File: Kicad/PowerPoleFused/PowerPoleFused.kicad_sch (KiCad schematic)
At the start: 6 parts, among them J1 Anderson powerpole, J2 Anderson powerpole, J3 Anderson powerpole, J4 Anderson powerpole, J5 Anderson powerpole, J6 Anderson powerpole

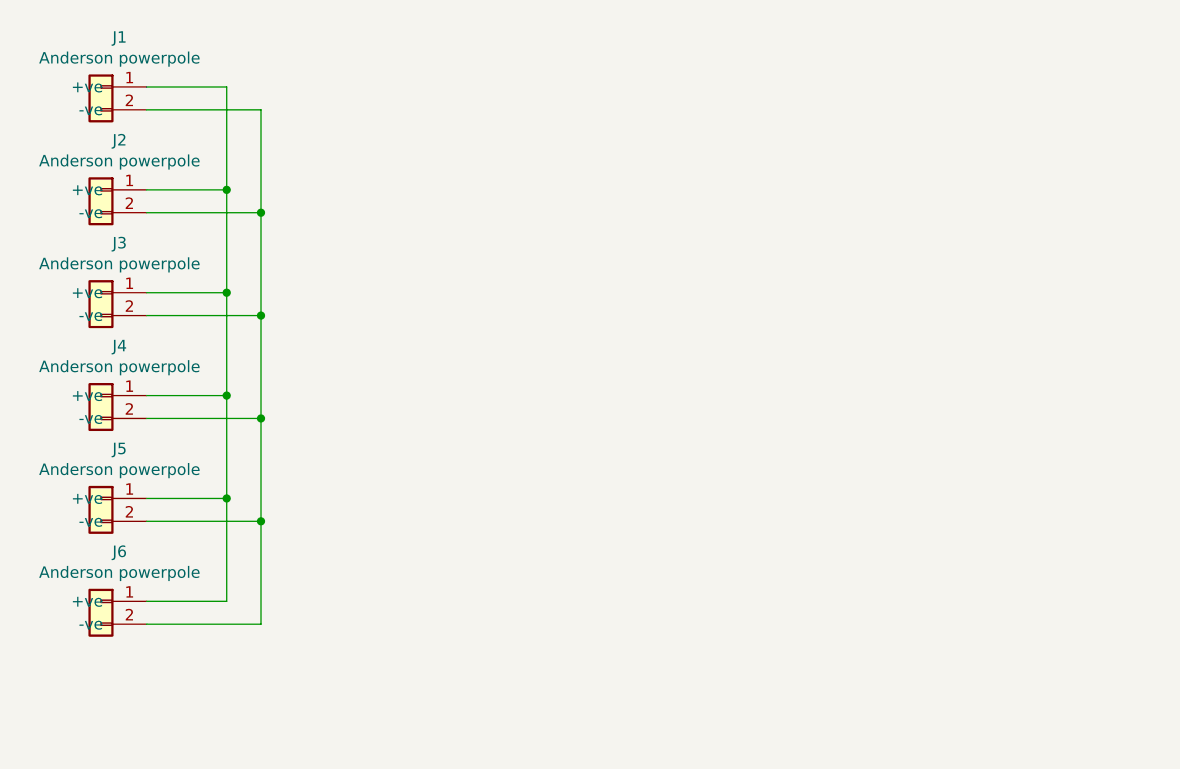
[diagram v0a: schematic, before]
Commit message: Laid out board 1st attempt
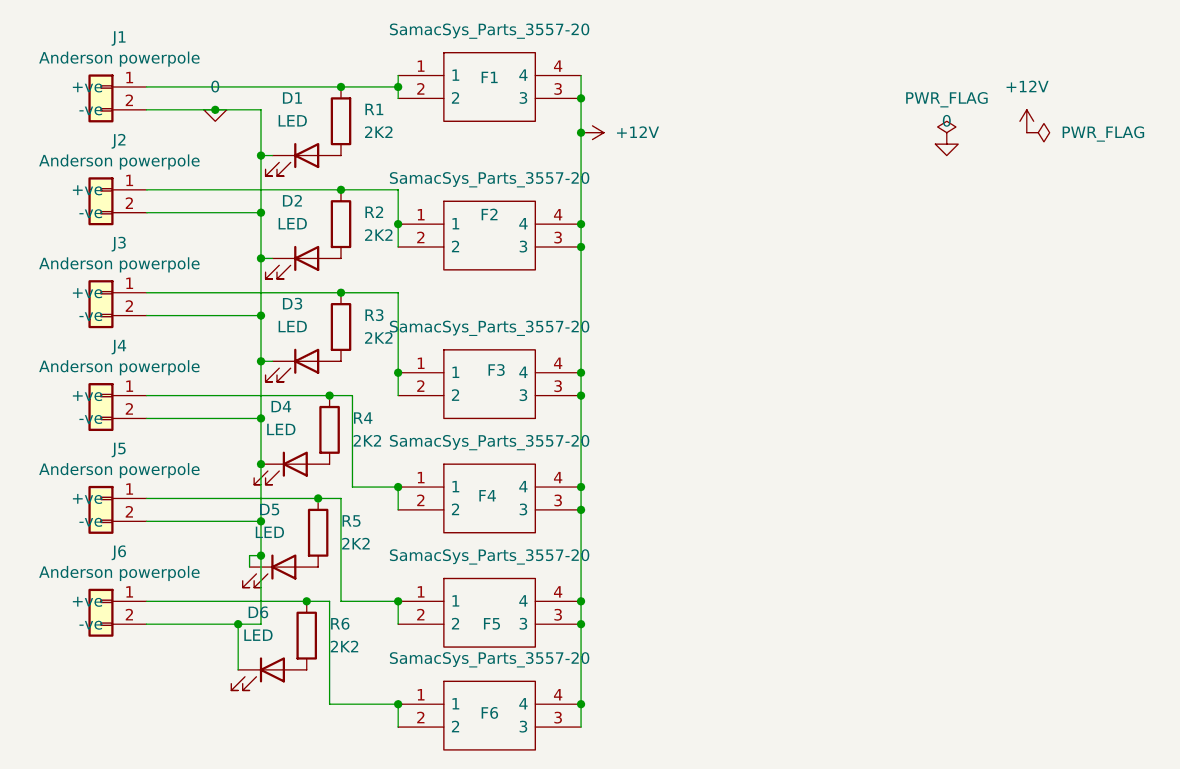
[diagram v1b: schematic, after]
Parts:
- added D1, D2, D3, D4, D5, D6: LED, LED_THT:LED_D5.0mm, symbol Device:LED
- added F1, F2, F3, F4, F5, F6: SamacSys_Parts_3557-20, Fuses:355720, symbol PowerPole-rescue:3557-20-SamacSys_Parts
- added R1, R2, R3, R4, R5, R6: 2K2, Resistor_THT:R_Axial_DIN0207_L6.3mm_D2.5mm_P7.62mm_Horizontal, symbol Device:R
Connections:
- net 0: now reaches J1.2 (-ve), J2.2 (-ve), J3.2 (-ve), J4.2 (-ve), J5.2 (-ve), J6.2 (-ve)
- net 0: now also D1.1 (K), D2.1 (K), D3.1 (K), D4.1 (K), D5.1 (K), D6.1 (K)
- new net: F1.1, F1.2, J1.1 (+ve), R1.2
- new net: F5.1, F5.2, J5.1 (+ve), R5.1
- new net: D5.2 (A), R5.2
- new net: F3.1, F3.2, J3.1 (+ve), R3.1
- new net: D4.2 (A), R4.2
- new net: F6.1, F6.2, J6.1 (+ve), R6.1
- new net: D6.2 (A), R6.2
- new net: F4.1, F4.2, J4.1 (+ve), R4.1
- new net: F2.1, F2.2, J2.1 (+ve), R2.1
- new net: D1.2 (A), R1.1
- new net: D3.2 (A), R3.2
- new net: D2.2 (A), R2.2
- new net +12V: F1.3, F1.4, F2.3, F2.4, F3.3, F3.4, F4.3, F4.4, F5.3, F5.4, F6.3, F6.4
